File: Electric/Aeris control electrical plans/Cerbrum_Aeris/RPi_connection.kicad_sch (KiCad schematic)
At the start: 1 part, among them J14 Raspberry_Pi_4

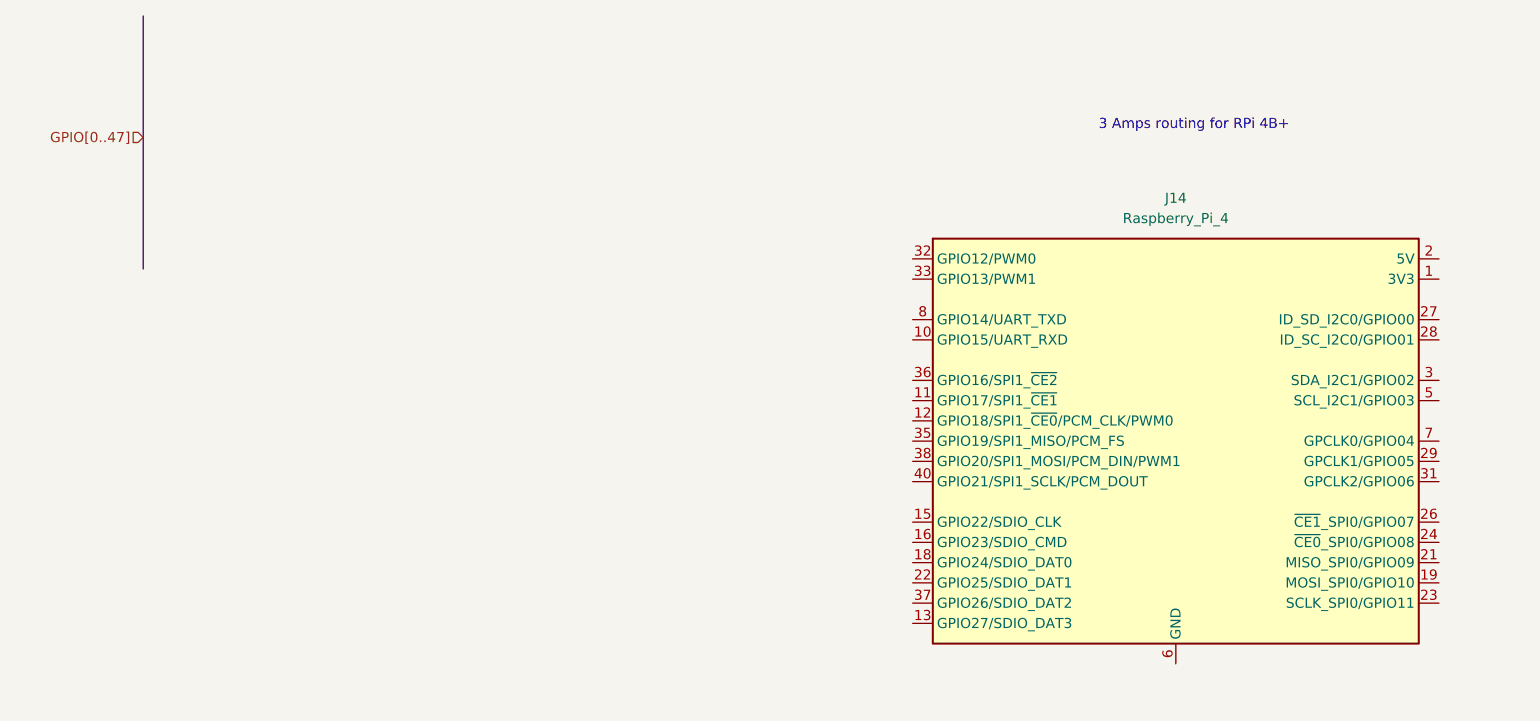
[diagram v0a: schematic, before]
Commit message: push éelectrique pcb
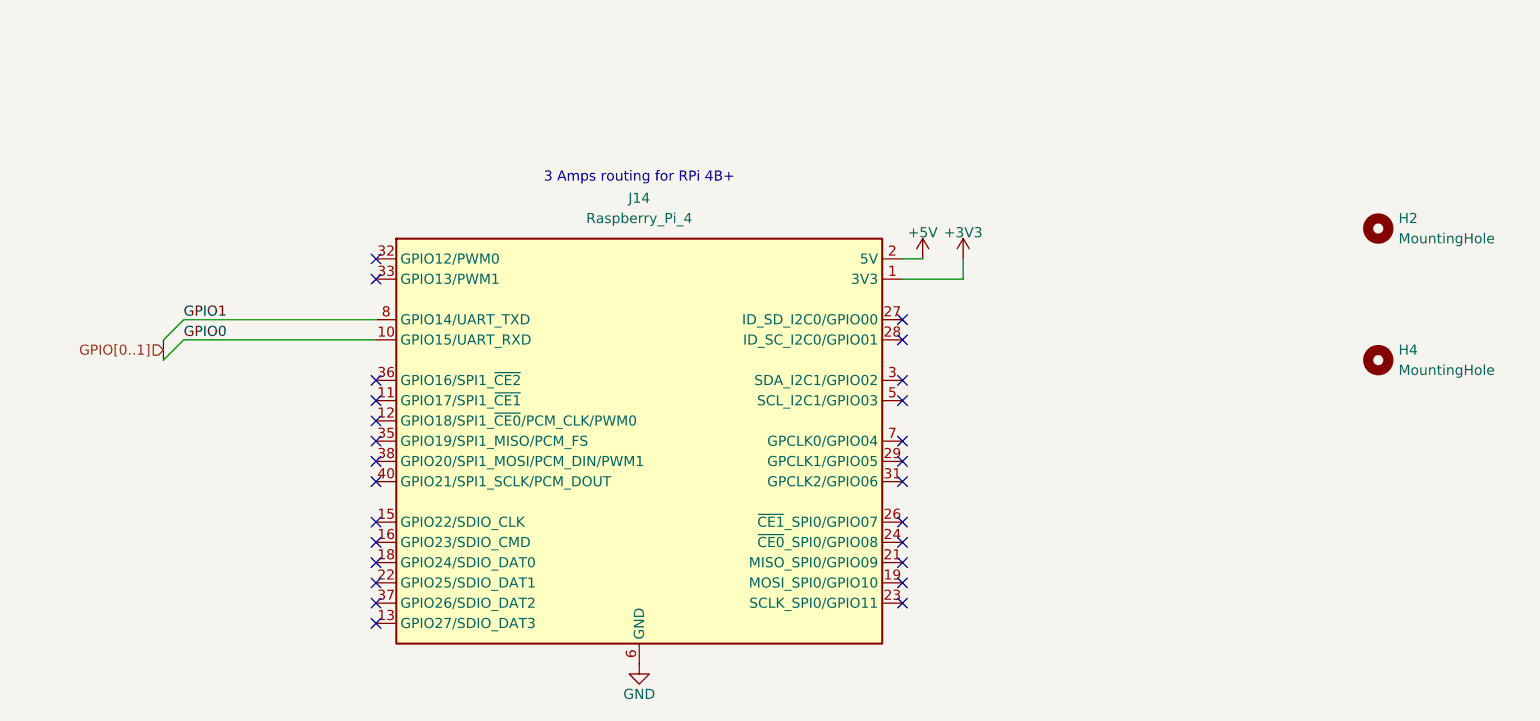
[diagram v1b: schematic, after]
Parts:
- added H2, H4: MountingHole, MountingHole:MountingHole_3.5mm, symbol Mechanical:MountingHole
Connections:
- net +3V3: now reaches J14.1 (3V3), J14.17 (3V3)
- net GPIO0: now reaches J14.10 (GPIO15/UART_RXD)
- net GND: now reaches J14.14 (GND), J14.20 (GND), J14.25 (GND), J14.30 (GND), J14.34 (GND), J14.39 (GND), J14.6 (GND), J14.9 (GND)
- net +5V: now reaches J14.2 (5V), J14.4 (5V)
- net GPIO1: now reaches J14.8 (GPIO14/UART_TXD)
- no-connect marks 0 -> 26
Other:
- moved on the sheet: J14
